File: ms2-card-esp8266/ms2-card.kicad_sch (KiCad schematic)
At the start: 56 parts, among them J1 Schaltregler, J10 MicroSD_SPI_CD, J11 Conn_01x06, J2 ESP Prog, J20 Smartcard Connector, J21 PogoPin, J22 Card Edge, J23 Conn_01x04, J30 USB_B_Micro, J31 Power Select, J32 Conn_01x03, Q1 MMBT3904, Q2 MMBT3904, SW1 RESET, U1 ESP-12F, U2 FM24C64B, U20 BL1551B, U3 BL1551B, U30 CP2102N-Axx-xQFN24, U4 BL1551B, U6 AMS1117-3.3

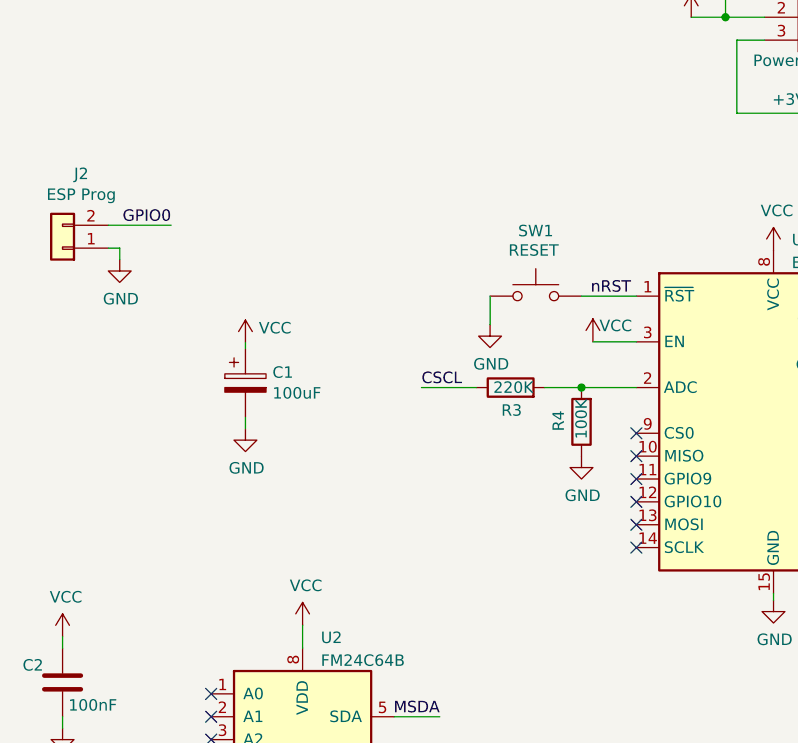
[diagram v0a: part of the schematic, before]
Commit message: add 3D pic
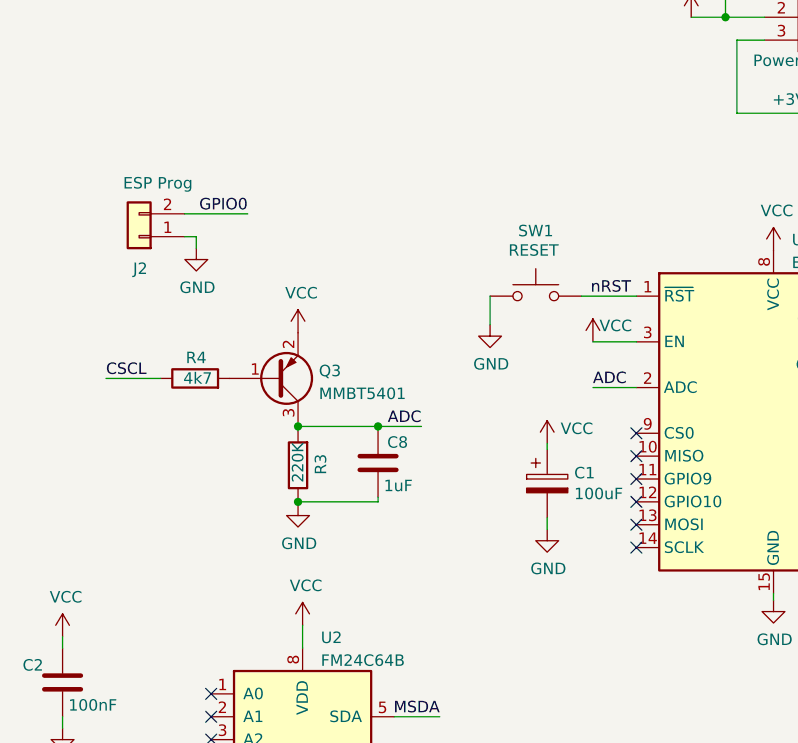
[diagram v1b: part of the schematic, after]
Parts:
- added C8: 1uF, Capacitor_SMD:C_0603_1608Metric, symbol Device:C
- added Q3: MMBT5401, Package_TO_SOT_SMD:SOT-23, symbol Transistor_BJT:MMBT3906
- R4: value 100K -> 4k7; LCSC C25803 -> C23162
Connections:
- net CSCL: now also R4.1; no longer R3.1
- net GND: now also R3.1, C8.2; no longer R4.1
- net VCC: now also Q3.2 (E)
- net ADC: now reaches R3.2, U1.2 (ADC)
- net ADC: now also C8.1, Q3.3 (C); no longer R4.2
- new net: Q3.1 (B), R4.2
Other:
- moved on the sheet: C1, J2, R3
